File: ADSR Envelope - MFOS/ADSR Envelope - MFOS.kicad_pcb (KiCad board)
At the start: 2 copper layers, 101.6 x 76.2 mm, 63 parts, among them J1 Trig_In, J10 SUS3, J12 Manual_Gate, J13 +12V_Conn, J14 -12V_Conn, J15 GND_Conn, J2 Gate_In, J3 APT, J4 RPT, J5 PCM, J6 DPT, J7 TSW, J8 SUS2, J9 ADSR, U1 4066, U2 TL082, U3 CD40106, U4 TL084, U5 4001

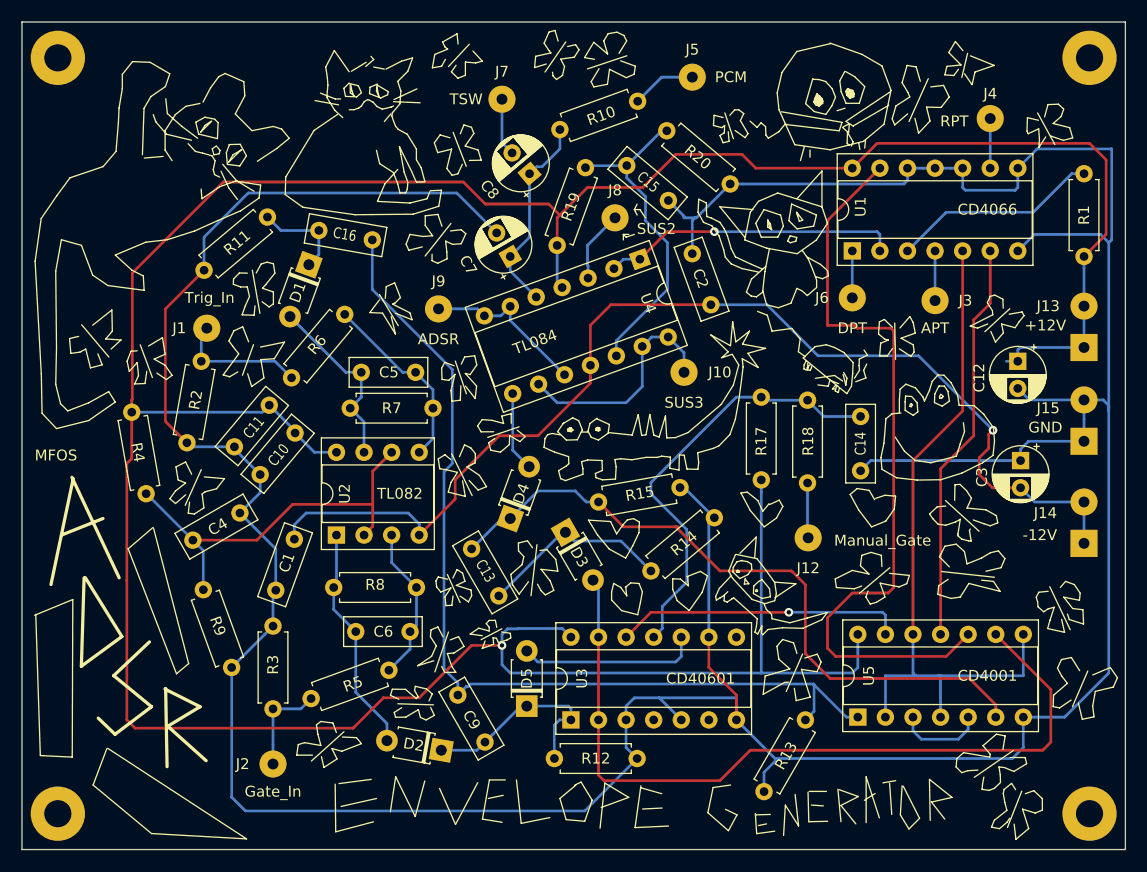
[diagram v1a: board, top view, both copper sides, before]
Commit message: hiiiii
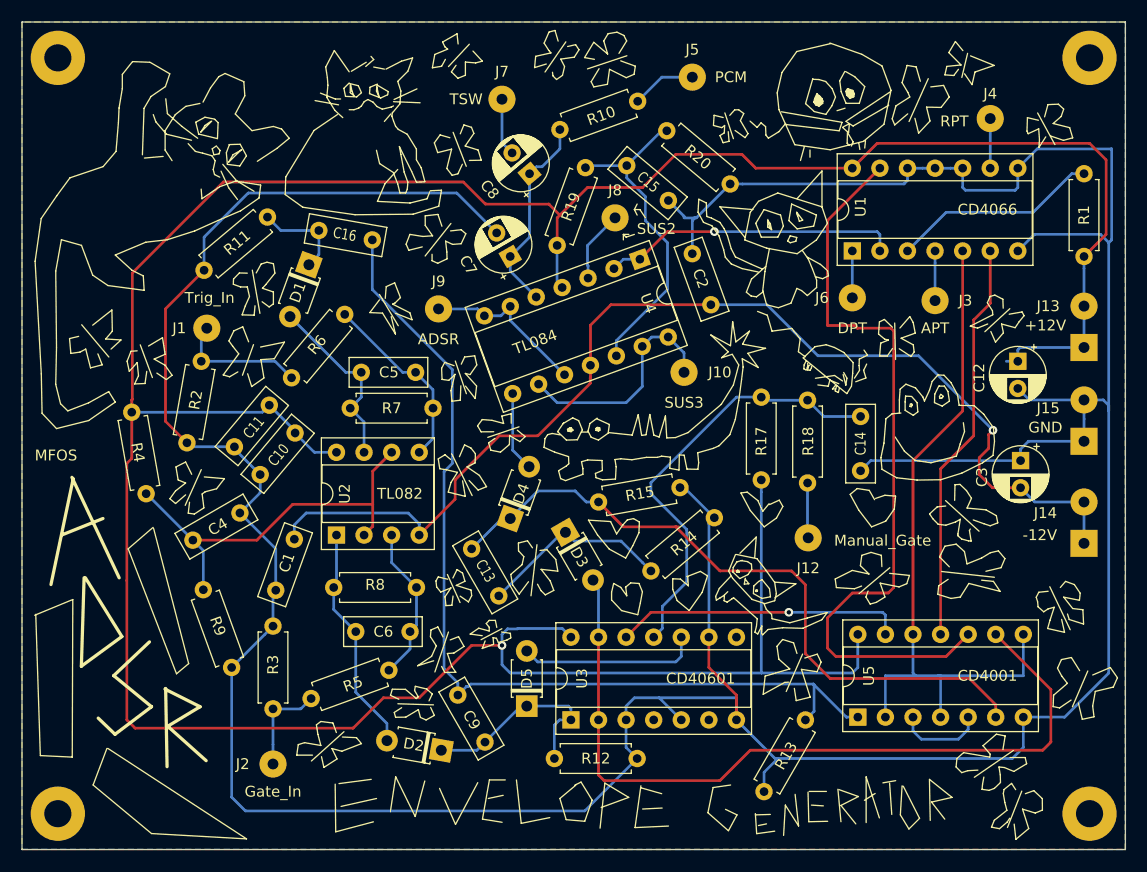
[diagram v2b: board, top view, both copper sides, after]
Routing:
- added copper zone on F.Cu, net (none)
- added copper zone on B.Cu, net Earth
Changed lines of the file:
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@@
   (page A4)
   (layers
-    (0 F.Cu signal)
+    (0 F.Cu signal hide)
     (31 B.Cu signal)
     (32 B.Adhes user hide)
@@
     (visible_elements FFFFFF7F)
     (pcbplotparams
-      (layerselection 0x010fc_ffffffff)
+      (layerselection 0x010e0_ffffffff)
       (usegerberextensions false)
       (usegerberattributes false)
@@
       (outputformat 1)
       (mirror false)
-      (drillshape 1)
+      (drillshape 0)
       (scaleselection 1)
       (outputdirectory ""))
@@
   (segment (start 94.234 77.47) (end 94.234 76.2) (width 0.25) (layer B.Cu) (net 40))
   (segment (start 94.996 78.232) (end 94.234 77.47) (width 0.25) (layer B.Cu) (net 40))
+  (zone (net 0) (net_name "") (layer F.Cu) (hatch edge 0.508)
+    (connect_pads (clearance 0.508))
+    (min_thickness 0.254)
+    (fill yes (arc_segments 32) (thermal_gap 0.508) (thermal_bridge_width 0.508))
+    (polygon
+      (pts
+        (xy 12.2 12.2) (xy 12.2 88.39) (xy 113.78 88.38) (xy 113.79 12.2)
+      )
+    )
+  )
+  (zone (net 1) (net_name Earth) (layer B.Cu) (hatch edge 0.508)
+    (connect_pads (clearance 0.508))
+    (min_thickness 0.254)
+    (fill yes (arc_segments 32) (thermal_gap 0.508) (thermal_bridge_width 0.508))
+    (polygon
+      (pts
+        (xy 12.2 12.2) (xy 12.2 88.37) (xy 113.79 88.39) (xy 113.79 12.19)
+      )
+    )
+  )
 )
